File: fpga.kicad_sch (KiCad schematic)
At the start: 6 parts, among them IC1 RP2040_breakout, J6 Micro_SD_Card, U3 CYC1000

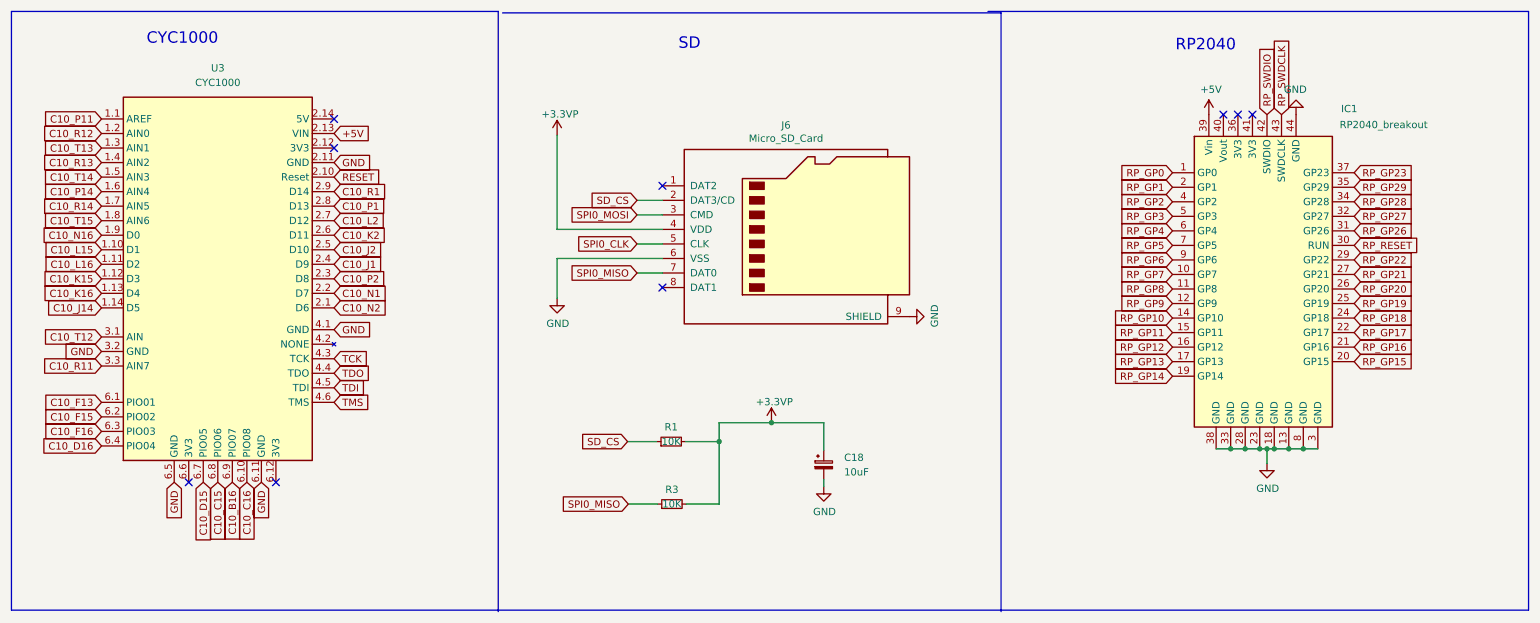
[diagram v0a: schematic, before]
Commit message: test
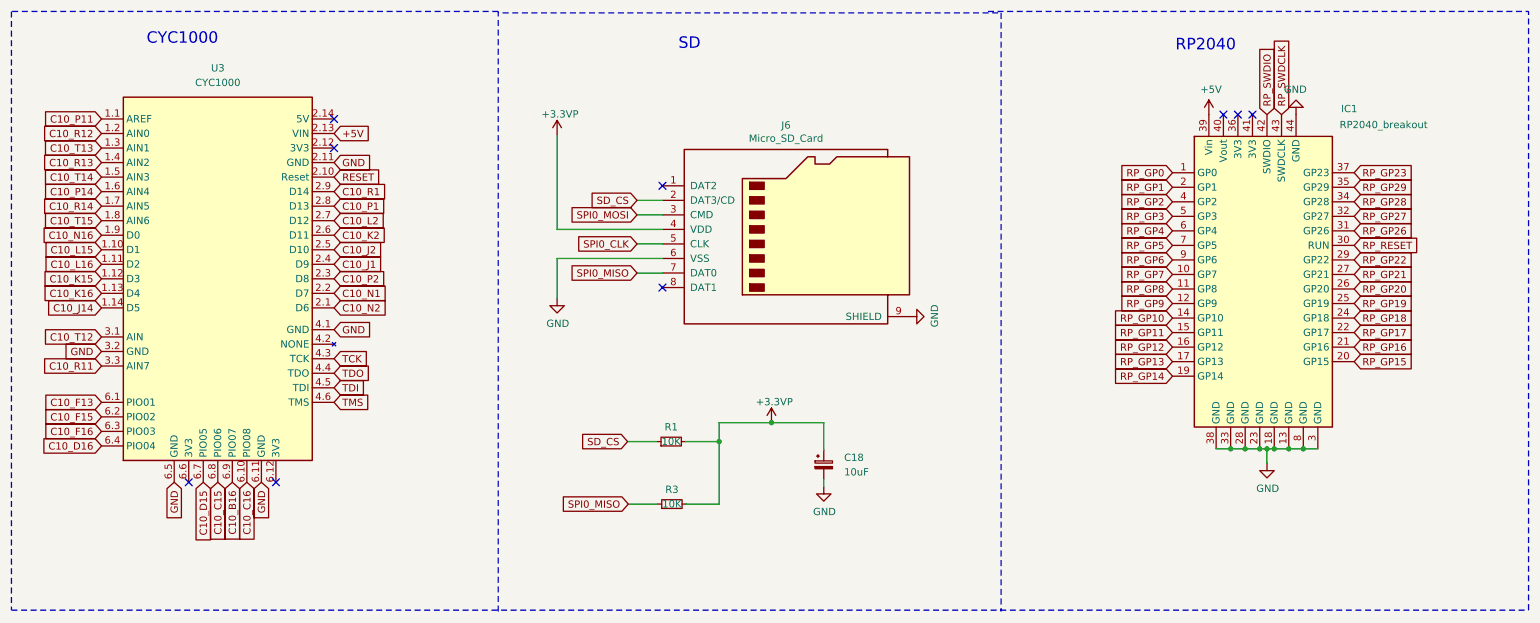
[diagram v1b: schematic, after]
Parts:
- C18: LCSC (none) -> C7171
- J6: LCSC (none) -> C585350
- R1, R3: footprint Resistor_SMD:R_1206_3216Metric_Pad1.30x1.75mm_HandSolder -> Resistor_SMD:R_0805_2012Metric_Pad1.20x1.40mm_HandSolder; LCSC (none) -> C17414
